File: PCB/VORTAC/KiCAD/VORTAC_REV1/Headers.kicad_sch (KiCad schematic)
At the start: 9 parts, among them J1 DEBUG, J14 918-418K2023S40001, J15 STEPPER, J3 Conn_01x05

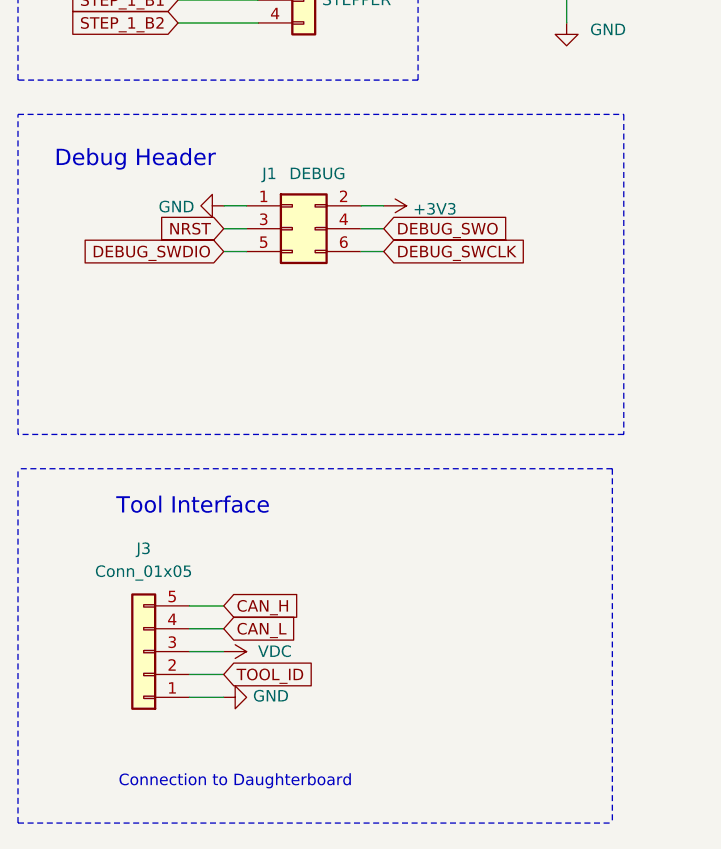
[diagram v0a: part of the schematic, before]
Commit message: BOMBOM
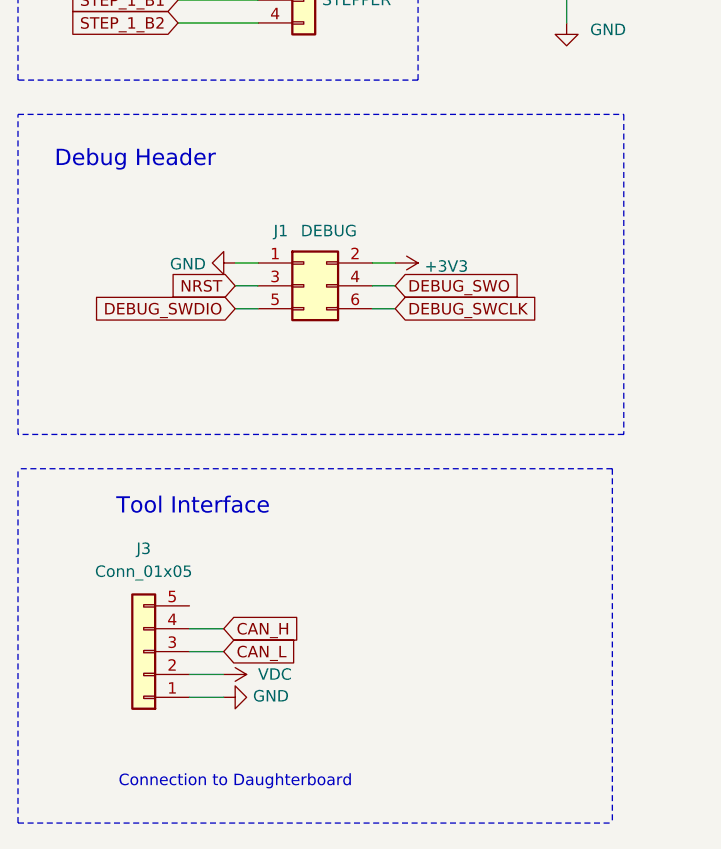
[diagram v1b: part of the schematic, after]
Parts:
- J1: footprint Vortac:PinHeader_2x03_P1.27mm_Vertical -> Connector_PinSocket_2.54mm:PinSocket_2x03_P2.54mm_Vertical
- J3: footprint Connector_PinHeader_2.54mm:PinHeader_2x03_P2.54mm_Vertical -> Connector_PinHeader_2.54mm:PinHeader_2x02_P2.54mm_Vertical
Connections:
- net TOOL_ID is gone; now on net VDC: J3.2 (Pin_2)
- net CAN_H: now also J3.4 (Pin_4); no longer J3.5 (Pin_5)
- net CAN_L: now also J3.3 (Pin_3); no longer J3.4 (Pin_4)
- net VDC: no longer J3.3 (Pin_3)
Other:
- moved on the sheet: J1

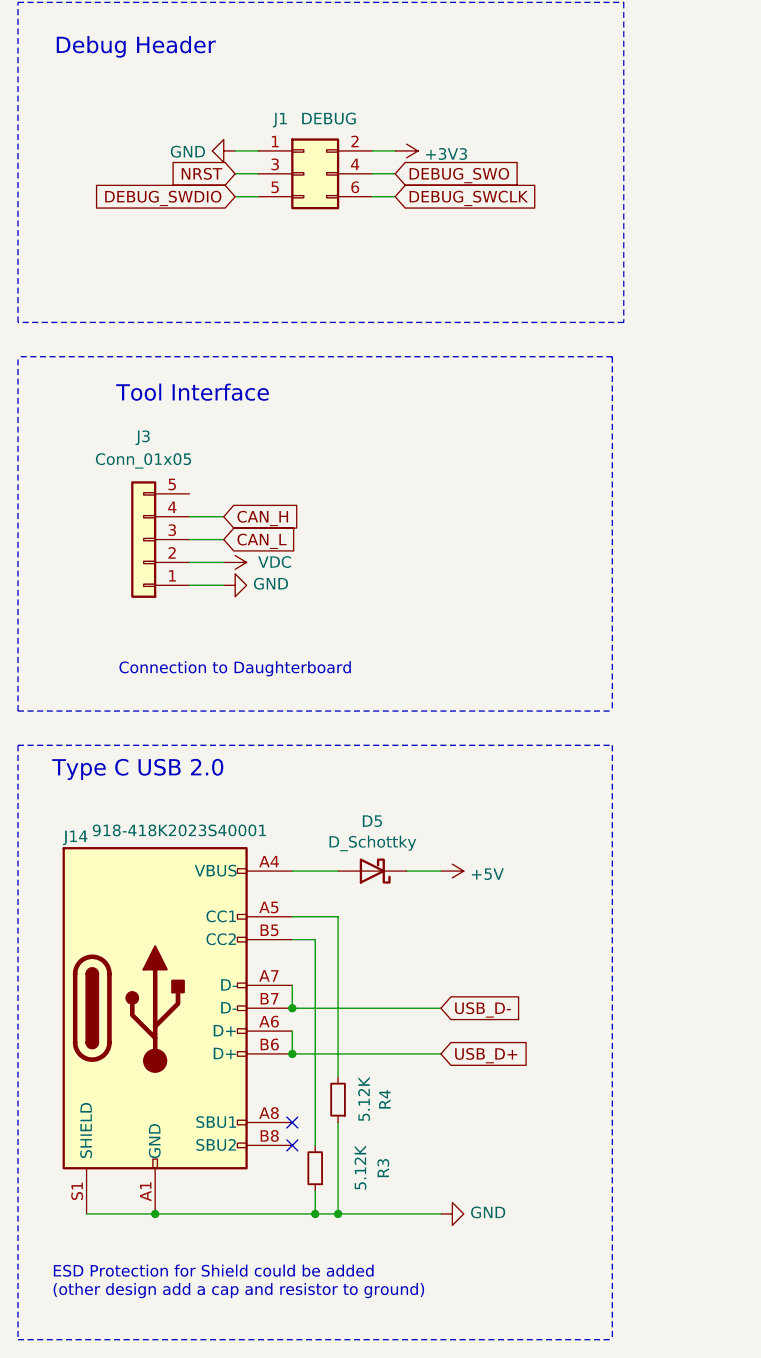
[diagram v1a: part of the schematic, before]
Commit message: Anned Parts
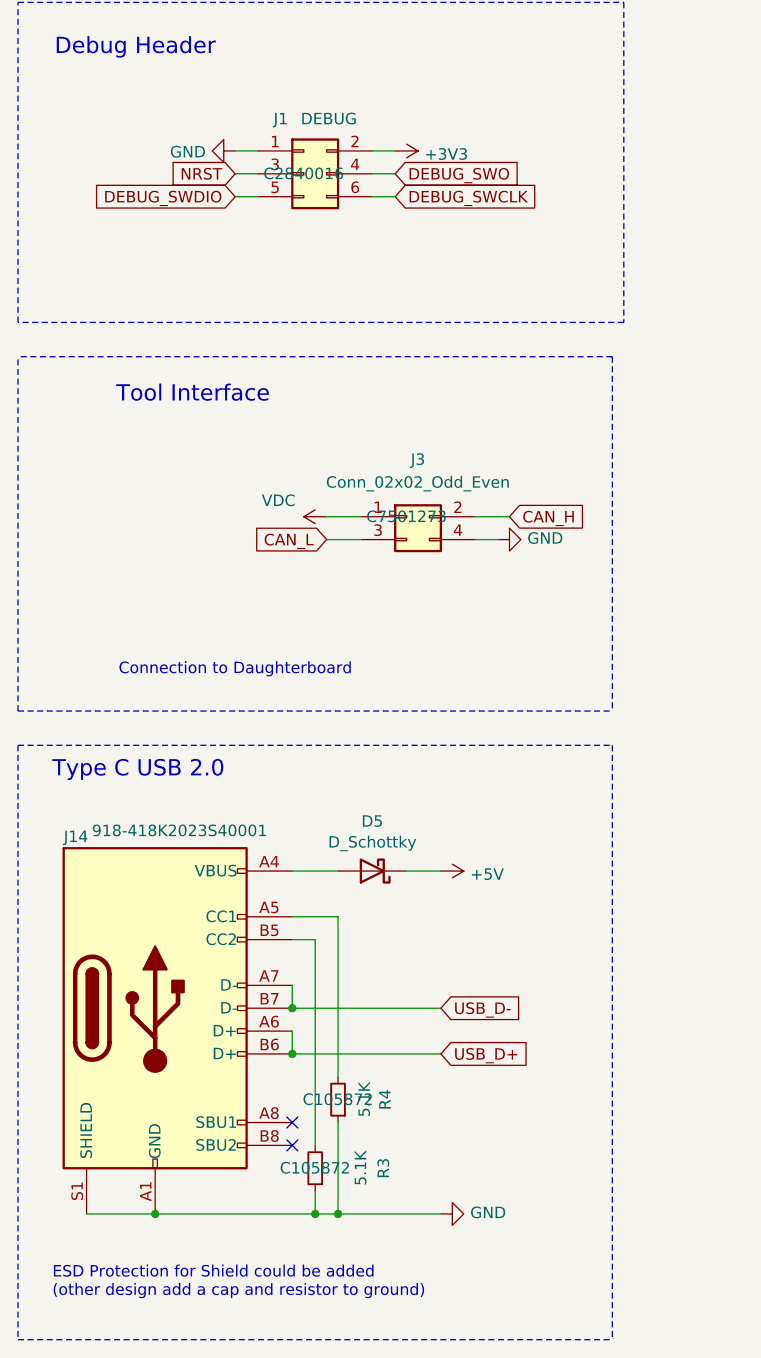
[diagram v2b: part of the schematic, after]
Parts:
- removed J3: Conn_01x05, Connector_PinHeader_2.54mm:PinHeader_2x02_P2.54mm_Vertical, symbol Connector_Generic:Conn_01x05
- added J3: Conn_02x02_Odd_Even, Connector_PinHeader_2.54mm:PinHeader_2x02_P2.54mm_Vertical, symbol Connector_Generic:Conn_02x02_Odd_Even
- D5: LCSC C37049 -> C7420331
- J1: LCSC (none) -> C2840016
- R3, R4: value 5.12K -> 5.1K; LCSC (none) -> C105872
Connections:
- net CAN_H: now also J3.2 (Pin_2)
- net CAN_L: now also J3.3 (Pin_3)
- net GND: now also J3.4 (Pin_4)
- net VDC: now also J3.1 (Pin_1)
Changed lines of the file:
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@@
-		)
-	)
-	(wire
-		(pts
-			(xy 35.56 101.6) (xy 39.37 101.6)
-		)
-		(stroke
-			(width 0)
-			(type default)
-		)
-	)
-	(wire
-		(pts
-			(xy 35.56 106.68) (xy 39.37 106.68)
-		)
-		(stroke
-			(width 0)
-			(type default)
 		)
 	)
@@
 	(wire
 		(pts
-			(xy 35.56 109.22) (xy 39.37 109.22)
+			(xy 50.8 104.14) (xy 54.61 104.14)
 		)
 		(stroke
@@
 	(wire
 		(pts
-			(xy 35.56 104.14) (xy 39.37 104.14)
-		)
-		(stroke
-			(width 0)
-			(type default)
-		)
-	)
-	(wire
-		(pts
 			(xy 52.07 179.07) (xy 52.07 168.91)
 		)
@@
 	(wire
 		(pts
+			(xy 71.12 101.6) (xy 67.31 101.6)
+		)
+		(stroke
+			(width 0)
+			(type default)
+		)
+	)
+	(wire
+		(pts
 			(xy 52.07 163.83) (xy 52.07 146.05)
 		)
@@
 	(wire
 		(pts
+			(xy 69.85 104.14) (xy 67.31 104.14)
+		)
+		(stroke
+			(width 0)
+			(type default)
+		)
+	)
+	(wire
+		(pts
 			(xy 43.18 63.5) (xy 40.64 63.5)
 		)
@@
 			(width 0)
 			(type dash)
+		)
+	)
+	(wire
+		(pts
+			(xy 50.8 101.6) (xy 54.61 101.6)
+		)
+		(stroke
+			(width 0)
+			(type default)
 		)
 	)
@@
 	(global_label "CAN_L"
 		(shape input)
-		(at 39.37 104.14 0)
+		(at 50.8 104.14 180)
 		(effects
 			(font
 				(size 1.27 1.27)
 			)
-			(justify left)
+			(justify right)
 		)
 		(property "Intersheetrefs" "${INTERSHEET_REFS}"
-			(at 39.37 104.14 0)
+			(at 50.8 104.14 0)
 			(effects
 				(font
@@
 	(global_label "CAN_H"
 		(shape input)
-		(at 39.37 101.6 0)
+		(at 71.12 101.6 0)
 		(effects
 			(font
@@
 		)
 		(property "Intersheetrefs" "${INTERSHEET_REFS}"
-			(at 39.37 101.6 0)
+			(at 71.12 101.6 0)
 			(effects
 				(font
@@
 			)
 		)
-		(property "Value" "5.12K"
+		(property "Value" "5.1K"
 			(at 54.61 173.99 90)
 			(effects
@@
 				)
 				(hide yes)
+			)
+		)
+		(property "LCSC" "C105872"
+			(at 49.53 173.99 0)
+			(effects
+				(font
+					(size 1.27 1.27)
+				)
 			)
 		)
@@
 			)
 		)
-		(property "Value" "5.12K"
+		(property "Value" "5.1K"
 			(at 55.0164 166.37 90)
 			(effects
@@
 				)
 				(hide yes)
+			)
+		)
+		(property "LCSC" "C105872"
+			(at 52.07 166.37 0)
+			(effects
+				(font
+					(size 1.27 1.27)
+				)
 			)
 		)
@@
 			)
 		)
-		(property "LCSC" "C37049"
+		(property "LCSC" "C7420331"
 			(at 55.88 140.97 0)
 			(effects
@@
 			)
 		)
+		(property "LCSC" "C2840016"
+			(at 48.26 63.5 0)
+			(effects
+				(font
+					(size 1.27 1.27)
+				)
+			)
+		)
 		(pin "3"
 		)
@@
 	(symbol
 		(lib_id "power:GND")
-		(at 39.37 109.22 90)
+		(at 69.85 104.14 90)
 		(unit 1)
 		(exclude_from_sim no)
@@
 		(dnp no)
 		(property "Reference" "#PWR120"
-			(at 45.72 109.22 0)
+			(at 76.2 104.14 0)
 			(effects
 				(font
@@
 		)
 		(property "Value" "GND"
-			(at 42.6212 109.093 90)
+			(at 73.1012 104.013 90)
 			(effects
 				(font
@@
 		)
 		(property "Footprint" ""
-			(at 39.37 109.22 0)
+			(at 69.85 104.14 0)
 			(effects
 				(font
@@
 		)
 		(property "Datasheet" ""
-			(at 39.37 109.22 0)
+			(at 69.85 104.14 0)
 			(effects
 				(font
@@
 		)
 		(property "Description" "Power symbol creates a global label with name \"GND\" , ground"
-			(at 39.37 109.22 0)
+			(at 69.85 104.14 0)
 			(effects
 				(font
@@
 	)
 	(symbol
-		(lib_id "Connector_Generic:Conn_01x05")
-		(at 30.48 104.14 180)
-		(unit 1)
-		(exclude_from_sim no)
-		(in_bom yes)
-		(on_board yes)
-		(dnp no)
-		(fields_autoplaced yes)
-		(property "Reference" "J3"
-			(at 30.48 92.71 0)
-			(effects
-				(font
-					(size 1.27 1.27)
-				)
-			)
-		)
-		(property "Value" "Conn_01x05"
-			(at 30.48 95.25 0)
-			(effects
-				(font
-					(size 1.27 1.27)
-				)
-			)
-		)
-		(property "Footprint" "Connector_PinHeader_2.54mm:PinHeader_2x02_P2.54mm_Vertical"
-			(at 30.48 104.14 0)
-			(effects
-				(font
-					(size 1.27 1.27)
-				)
-				(hide yes)
-			)
-		)
-		(property "Datasheet" "~"
-			(at 30.48 104.14 0)
-			(effects
-				(font
-					(size 1.27 1.27)
-				)
-				(hide yes)
-			)
-		)
-		(property "Description" "Generic connector, single row, 01x05, script generated (kicad-library-utils/schlib/autogen/connector/)"
-			(at 30.48 104.14 0)
-			(effects
-				(font
-					(size 1.27 1.27)
-				)
-				(hide yes)
-			)
-		)
-		(pin "5"
-		)
-		(pin "2"
-		)
-		(pin "3"
-		)
-		(pin "1"
-		)
-		(pin "4"
-		)
-		(instances
-			(project "VORTAC_REV1"
-				(path "/ed58d858-d9f9-4504-a982-ccfc7f9efbad/00000000-0000-0000-0000-0000613db78d"
-					(reference "J3")
-					(unit 1)
-				)
-			)
-		)
-	)
-	(symbol
 		(lib_id "power:GND")
 		(at 40.64 60.96 270)
@@
 	)
 	(symbol
-		(lib_id "power:VDC")
-		(at 39.37 106.68 270)
+		(lib_id "Connector_Generic:Conn_02x02_Odd_Even")
+		(at 59.69 101.6 0)
 		(unit 1)
 		(exclude_from_sim no)
@@
 		(dnp no)
 		(fields_autoplaced yes)
+		(property "Reference" "J3"
+			(at 60.96 95.25 0)
+			(effects
+				(font
+					(size 1.27 1.27)
+				)
+			)
+		)
+		(property "Value" "Conn_02x02_Odd_Even"
+			(at 60.96 97.79 0)
+			(effects
+				(font
+					(size 1.27 1.27)
+				)
+			)
+		)
+		(property "Footprint" "Connector_PinHeader_2.54mm:PinHeader_2x02_P2.54mm_Vertical"
+			(at 59.69 101.6 0)
+			(effects
+				(font
+					(size 1.27 1.27)
+				)
+				(hide yes)
+			)
+		)
+		(property "Datasheet" "~"
+			(at 59.69 101.6 0)
+			(effects
+				(font
+					(size 1.27 1.27)
+				)
+				(hide yes)
+			)
+		)
+		(property "Description" "Generic connector, double row, 02x02, odd/even pin numbering scheme (row 1 odd numbers, row 2 even numbers), script generated (kicad-library-utils/schlib/autogen/connector/)"
+			(at 59.69 101.6 0)
+			(effects
+				(font
+					(size 1.27 1.27)
+				)
+				(hide yes)
+			)
+		)
+		(property "LCSC" "C7501273"
+			(at 59.69 101.6 0)
+			(effects
+				(font
+					(size 1.27 1.27)
+				)
+			)
+		)
+		(pin "1"
+		)
+		(pin "3"
+		)
+		(pin "4"
+		)
+		(pin "2"
+		)
+		(instances
+			(project ""
+				(path "/ed58d858-d9f9-4504-a982-ccfc7f9efbad/00000000-0000-0000-0000-0000613db78d"
+					(reference "J3")
+					(unit 1)
+				)
+			)
+		)
+	)
+	(symbol
+		(lib_id "power:VDC")
+		(at 50.8 101.6 90)
+		(unit 1)
+		(exclude_from_sim no)
+		(in_bom yes)
+		(on_board yes)
+		(dnp no)
 		(property "Reference" "#PWR1"
-			(at 35.56 106.68 0)
+			(at 54.61 101.6 0)
 			(effects
 				(font
@@
 		)
 		(property "Value" "VDC"
-			(at 43.18 106.6799 90)
-			(effects
-				(font
-					(size 1.27 1.27)
-				)
-				(justify left)
+			(at 45.466 99.822 90)
+			(effects
+				(font
+					(size 1.27 1.27)
+				)
 			)
 		)
 		(property "Footprint" ""
-			(at 39.37 106.68 0)
+			(at 50.8 101.6 0)
 			(effects
 				(font
@@
 		)
 		(property "Datasheet" ""
-			(at 39.37 106.68 0)
+			(at 50.8 101.6 0)
 			(effects
 				(font
@@
 		)
 		(property "Description" "Power symbol creates a global label with name \"VDC\""
-			(at 39.37 106.68 0)
-			(effects
-				(font
+			(at 50.8 101.6 0)
+			(effects
+				(font
